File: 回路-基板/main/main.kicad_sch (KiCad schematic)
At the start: 51 parts, among them J1 Conn_01x07_Pin, J2 Conn_01x08_Pin, J3 Conn_01x08_Pin, J4 Conn_01x08_Pin, J5 Conn_01x08_Pin, SW1 SW_Push, SW2 SW_Push, SW3 SW_Push, SW4 SW_Push, SW5 SW_Push, SW6 SW_Push, SW7 SW_Push, SW8 SW_SPDT, U1 TWE-L-WX, U2 LM1117MP-3.3

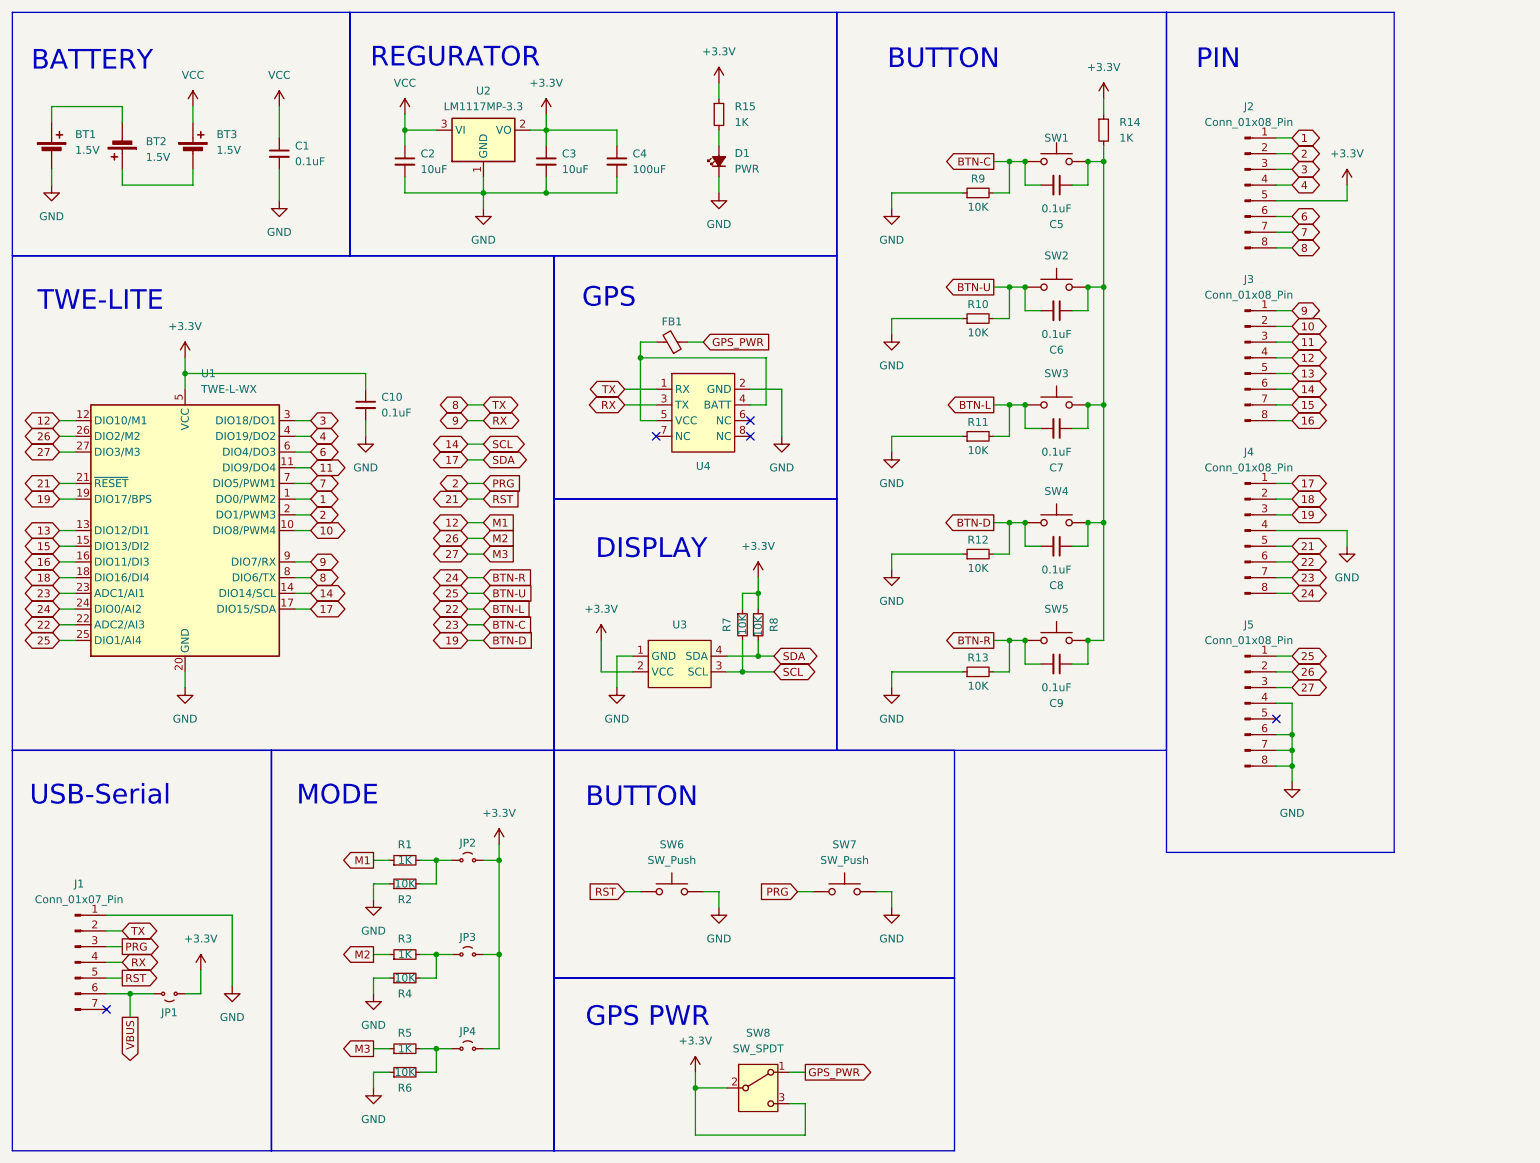
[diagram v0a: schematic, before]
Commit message: ピンのテストプログラムと基板の更新版PCB
PCBのDRよろしくー
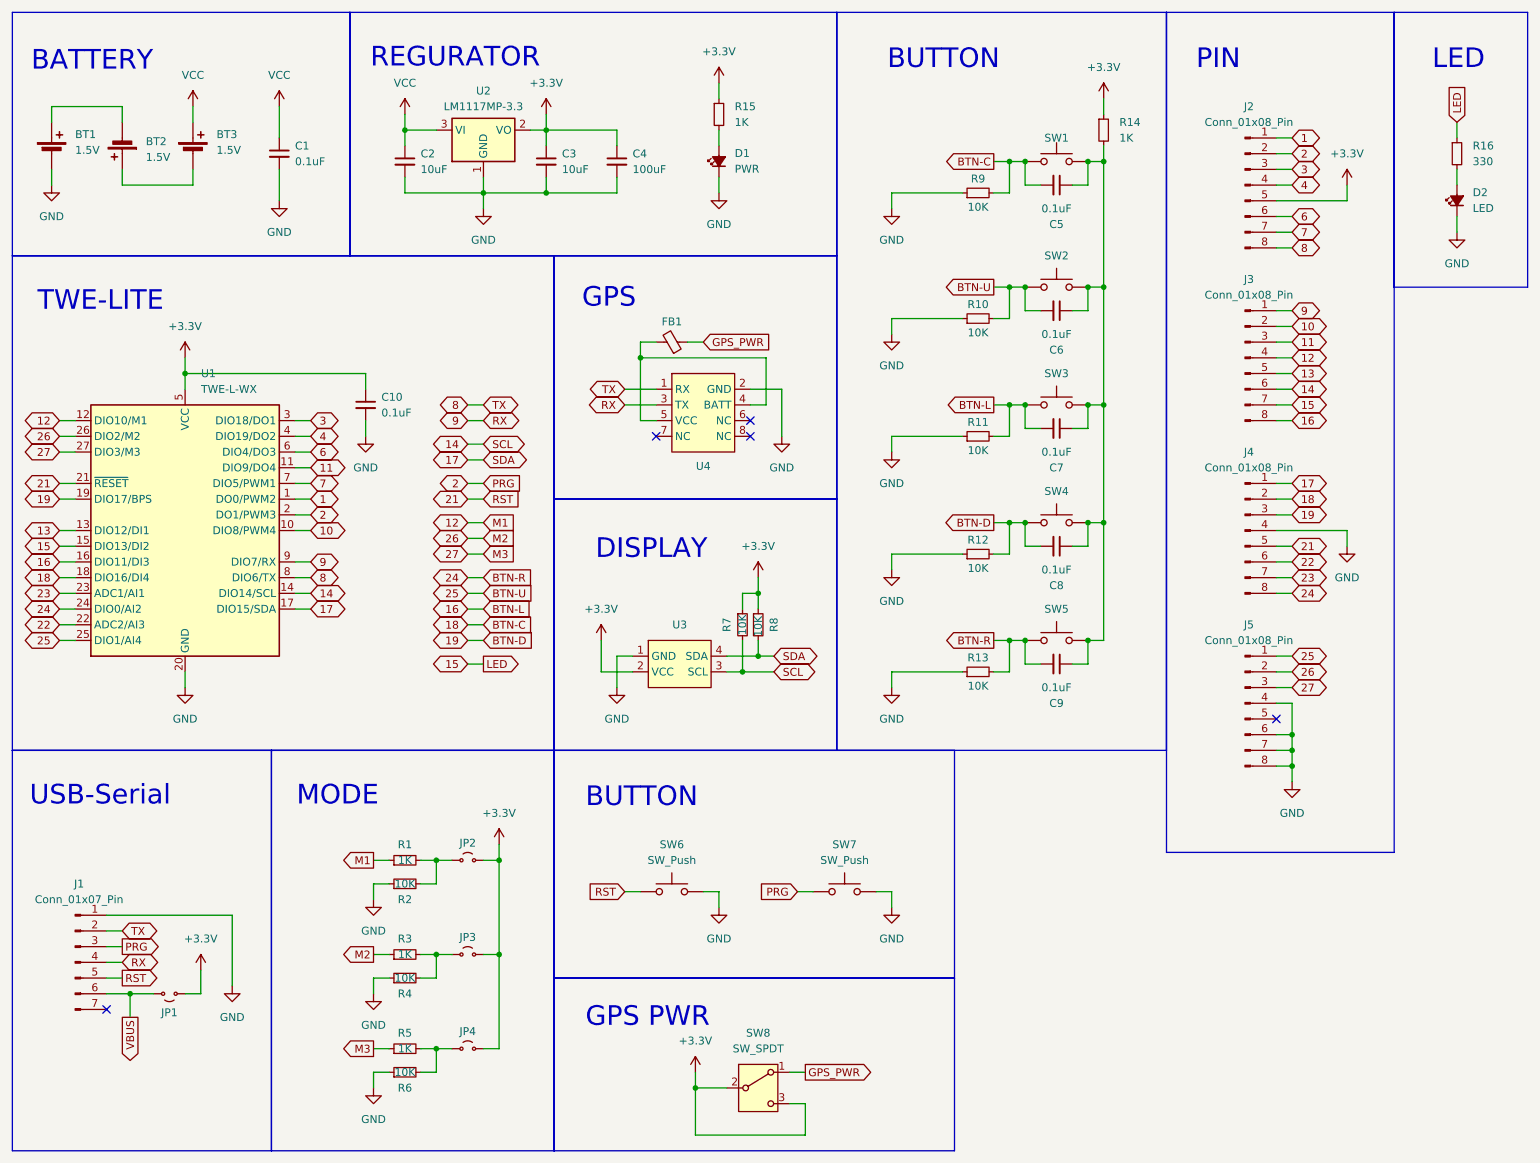
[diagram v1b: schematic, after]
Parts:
- added D2: LED, LED_SMD:LED_0805_2012Metric, symbol Device:LED_Small_Filled
- added R16: 330, Resistor_SMD:R_0805_2012Metric, symbol Device:R_Small
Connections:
- net 15: now also R16.1
- net 16: now also C7.2, R11.2, SW3.1
- net 18: now also C5.2, R9.2, SW1.1
- net 22: no longer C7.2, R11.2, SW3.1
- net 23: no longer C5.2, R9.2, SW1.1
- net GND: now also D2.1 (K)
- new net: D2.2 (A), R16.2
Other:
- note added: "LED"
